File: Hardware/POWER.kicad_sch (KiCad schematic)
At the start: 63 parts, among them J15 5V_USB, J17 Battery IN, Q1 RE1C002UN, U11 AOZ1212AI, U5 AP2112K-3.3, U5 AP2151W, U6 AP2112K-1.8, U7 AP2112K-3.3

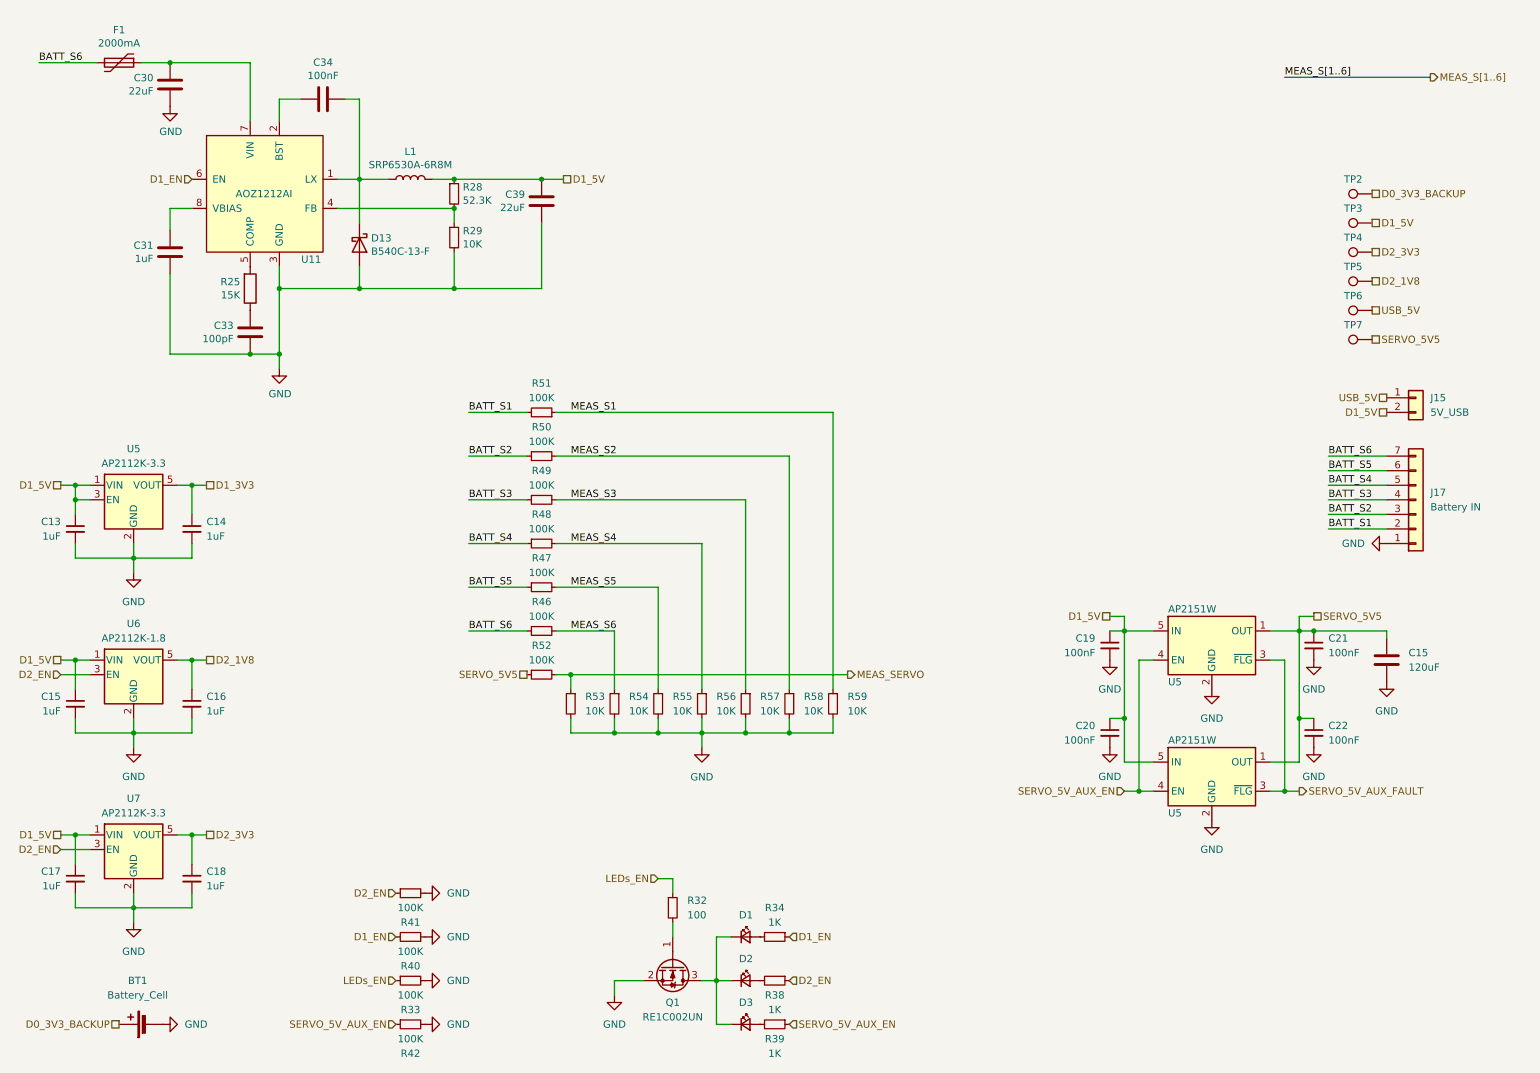
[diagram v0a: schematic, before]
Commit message: Checkpoint
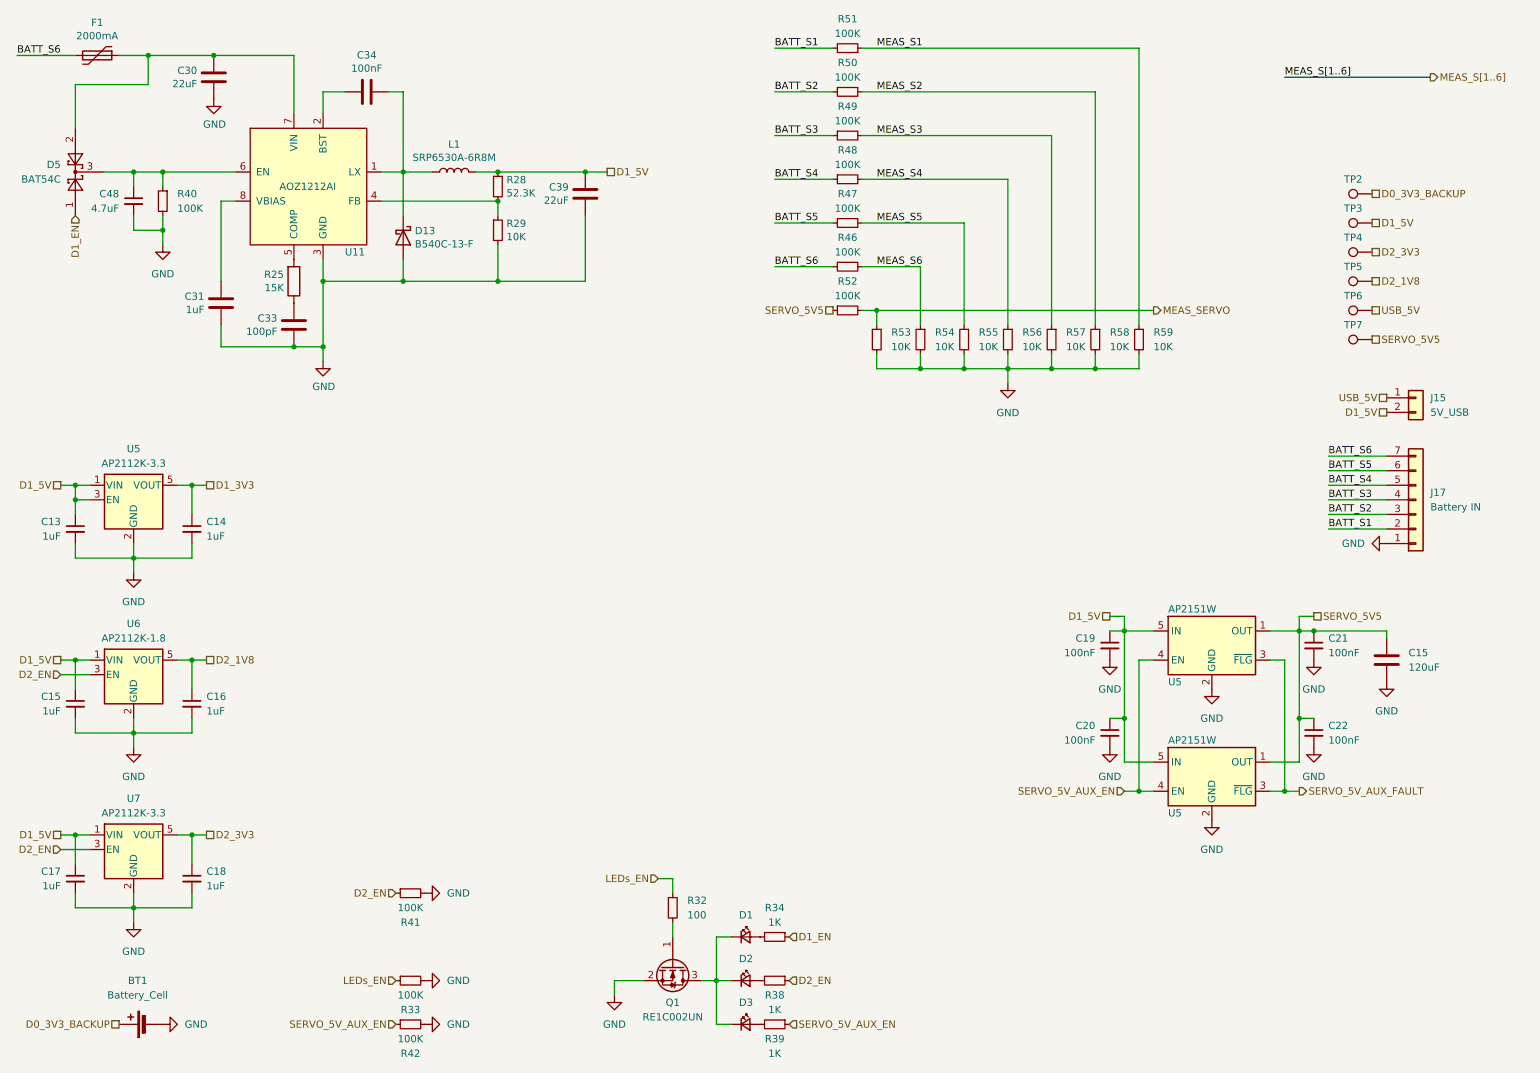
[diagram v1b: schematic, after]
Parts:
- added C48: 4.7uF, symbol Device:C_Small
- added D5: BAT54C, Package_TO_SOT_SMD:SOT-23, symbol Diode:BAT54C
- C33, C34: footprint Capacitor_SMD:C_0805_2012Metric -> (none)
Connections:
- net D1_EN: now also D5.1; no longer R40.2, U11.6 (EN)
- net GND: now also R40.2, C48.2; no longer R40.1
- net at C30.2, F1.1, U11.7 (VIN): now also D5.2
- new net: C48.1, D5.3, R40.1, U11.6 (EN)
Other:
- moved on the sheet: C30, C31, C33, C34, C39, D13, F1, L1, R25, R28, R29, R40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
